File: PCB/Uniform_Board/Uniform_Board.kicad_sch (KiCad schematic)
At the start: 140 parts, among them J1 PCIE_x1_SAMTEC_PCIE-036-02-F-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

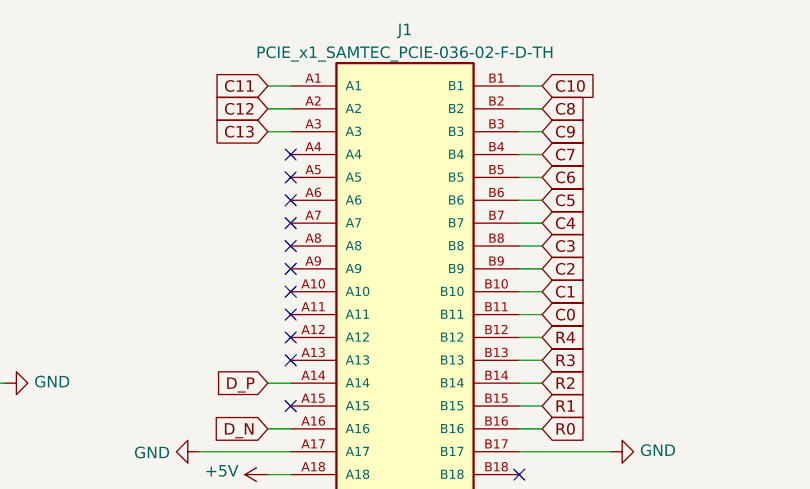
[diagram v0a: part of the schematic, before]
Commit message: started board routing; first attempt
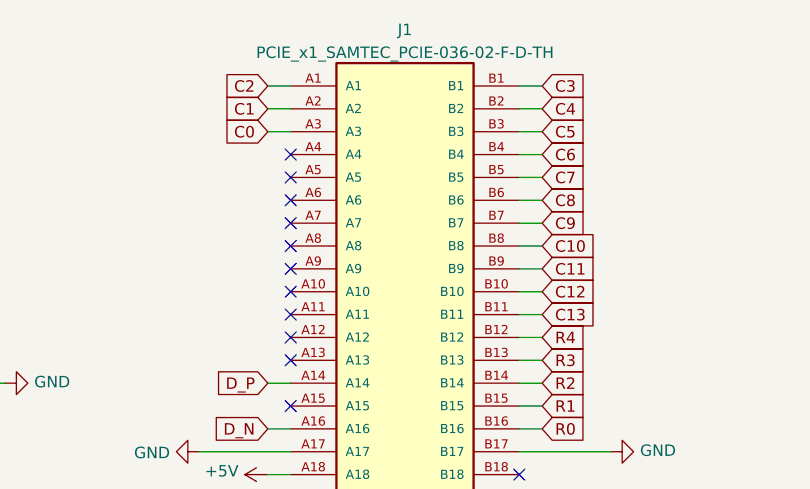
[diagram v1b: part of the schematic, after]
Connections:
- net C0: now also J1.A3; no longer J1.B11
- net C1: now also J1.A2; no longer J1.B10
- net C10: now also J1.B8; no longer J1.B1
- net C11: now also J1.B9; no longer J1.A1
- net C12: now also J1.B10; no longer J1.A2
- net C13: now also J1.B11; no longer J1.A3
- net C2: now also J1.A1; no longer J1.B9
- net C3: now also J1.B1; no longer J1.B8
- net C4: now also J1.B2; no longer J1.B7
- net C5: now also J1.B3; no longer J1.B6
- net C6: now also J1.B4; no longer J1.B5
- net C7: now also J1.B5; no longer J1.B4
- net C8: now also J1.B6; no longer J1.B2
- net C9: now also J1.B7; no longer J1.B3
